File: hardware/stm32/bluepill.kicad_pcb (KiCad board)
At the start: 2 copper layers, 99.1 x 99.1 mm, 71 parts, among them J1 LCD, J10 Screw_Terminal_01x02, J11 Screw_Terminal_01x02, J12 Screw_Terminal_01x02, J13 Screw_Terminal_01x02, J14 RTC, J15 Screw_Terminal_01x02, J16 Conn_01x02_Male, J17 ESP-01, J18 USART1, J19 Buttons, J2 SD Card, J3 Radio, J4 Inside, J5 Outside, J6 Screw_Terminal_01x02, J7 Conn_01x02, J8 Screw_Terminal_01x02, J9 Screw_Terminal_01x02, Q1 Q_NMOS_GSD, Q2 Q_NMOS_GSD, Q3 Q_NMOS_GSD, Q4 Q_NMOS_GSD, Q5 Q_NMOS_GSD, Q6 Q_NMOS_GSD, U1 PC817, U10 PC817, U11 PC817, U12 LM1117-3.3, U2 24LC512, U3 bluepill, U4 PC817, U5 PC817, U6 PC817, U7 PC817, U8 PC817, U9 PC817

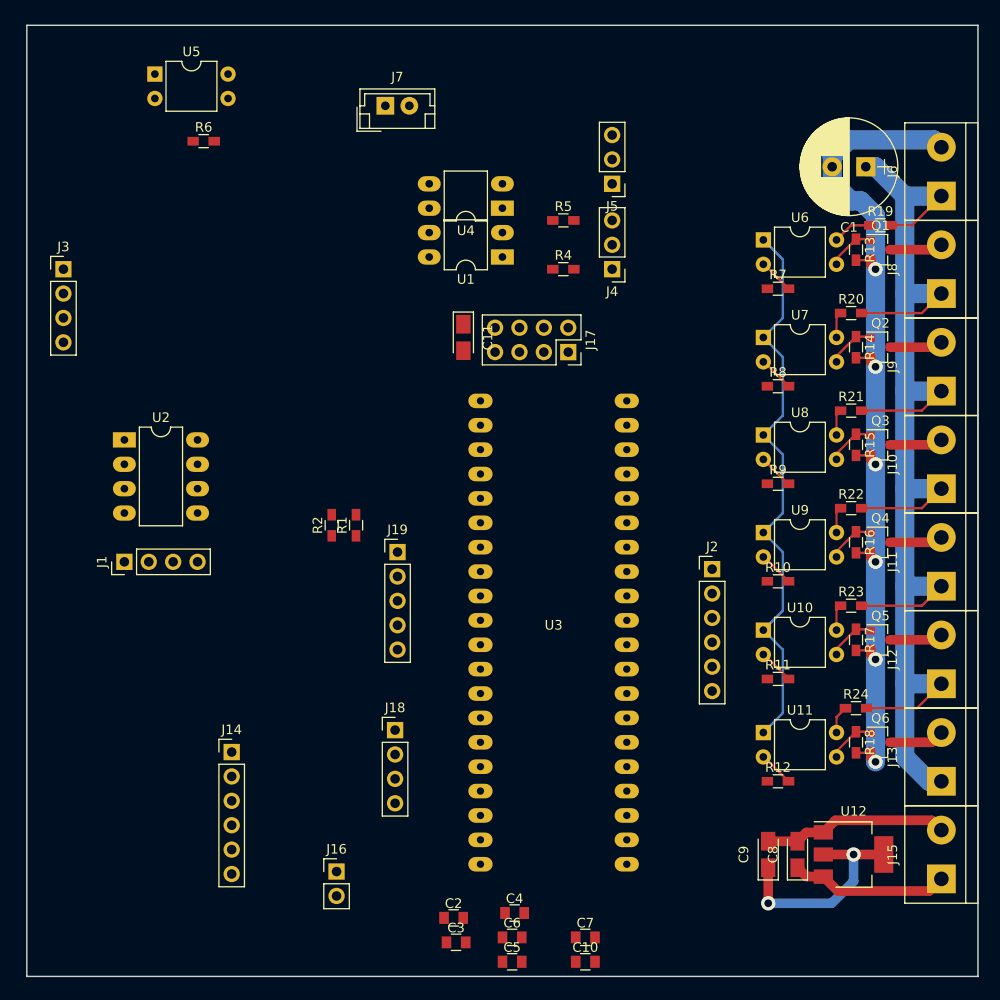
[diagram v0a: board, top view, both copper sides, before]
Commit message: bluepill PCB progress
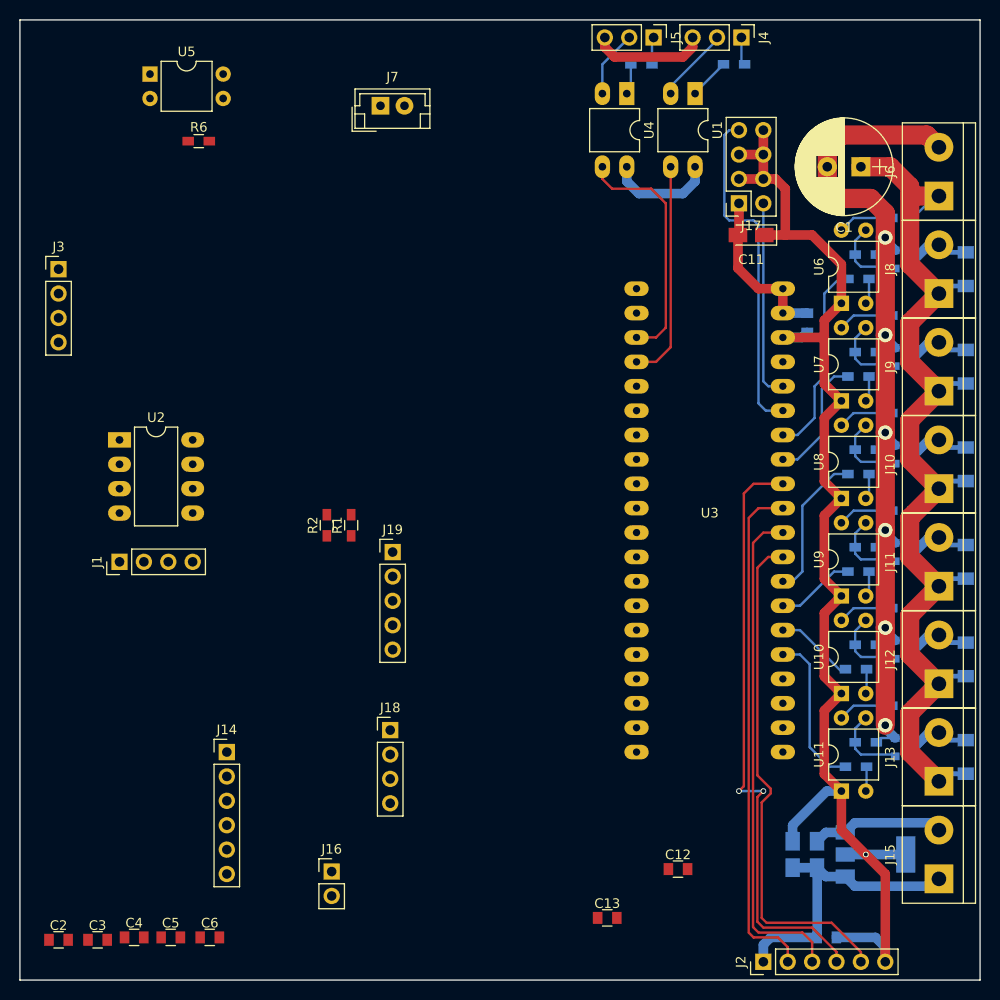
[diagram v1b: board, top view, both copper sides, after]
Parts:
- added C12: 100n, Capacitors_SMD:C_0805, F.Cu at (113.5, 123.4)
- added C13: 100n, Capacitors_SMD:C_0805, F.Cu at (106.2, 128.5)
- added D1: 1N4148, Diodes_SMD:D_MiniMELF, B.Cu at (143.5, 61.0)
- added D2: 1N4148, Diodes_SMD:D_MiniMELF, B.Cu at (143.5, 71.1)
- added D3: 1N4148, Diodes_SMD:D_MiniMELF, B.Cu at (143.5, 81.3)
- added D4: 1N4148, Diodes_SMD:D_MiniMELF, B.Cu at (143.5, 91.4)
- added D5: 1N4148, Diodes_SMD:D_MiniMELF, B.Cu at (143.5, 101.6)
- added D6: 1N4148, Diodes_SMD:D_MiniMELF, B.Cu at (143.5, 111.8)
- C10, C7, C8, C9, R10, R11, R12, R13, R14, R15, R16, R17, R18, R19, R20, R21, R22, R23, R24, R4, R5, R7, R8, R9, U12: moved to B.Cu
- J15: value Screw_Terminal_01x02 -> +5V
- Q1, Q2, Q3, Q4, Q5, Q6: value Q_NMOS_GSD -> IRLML2502; moved to B.Cu
- moved C7 68.1 mm to (127.0, 66.5), turned to 90 degrees
- moved J2 41.2 mm to (122.4, 133.1), turned to 90 degrees
- moved C2 41.2 mm to (49.0, 130.8)
- moved C4 39.7 mm to (56.9, 130.6)
- moved C3 37.3 mm to (53.1, 130.8)
- moved C5 35.7 mm to (60.7, 130.6)
- moved C11 31.8 mm to (121.2, 57.4), turned to 180 degrees
- moved C6 31.5 mm to (64.8, 130.6)
- moved R4 27.8 mm to (119.4, 39.6)
- moved J4 27.6 mm to (120.1, 36.8), turned to 270 degrees
- moved U1 26.3 mm to (115.3, 42.7), turned to 270 degrees
- moved C10 25.3 mm to (129.0, 130.6), turned to 180 degrees
- moved J17 23.6 mm to (119.9, 54.1), turned to 180 degrees
- moved U3 20.0 mm to (116.8, 85.9)
- moved R5 18.2 mm to (109.7, 39.6)
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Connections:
- J15 pad 1: +5V -> GND
- J15 pad 2: GND -> +5V
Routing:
- net +3V3: track 82.4 -> 148.7 mm, vias 2 -> 1
- net /MCU/MOSI: track 0.00 -> 62.7 mm, vias 0 -> 2
- net /MCU/MISO: track 0.00 -> 53.4 mm
- net /MCU/CS: track 0.00 -> 53.4 mm
- net /MCU/SCK: track 0.00 -> 52.4 mm
- net GND: track 19.4 -> 60.8 mm
- net /MCU/ESP_RX: track 0.00 -> 35.5 mm
- net /MCU/LOOP_O: track 0.00 -> 25.3 mm
- net /MCU/LOOP_I: track 0.00 -> 23.0 mm
- net Net-(R7-Pad1): track 0.00 -> 21.5 mm
- net /MCU/ESP_TX: track 0.00 -> 20.8 mm
- net +12V: track 143.4 -> 126.5 mm
- net Net-(R12-Pad1): track 0.00 -> 16.4 mm
- net Net-(R9-Pad1): track 0.00 -> 15.4 mm
- net Net-(R8-Pad1): track 0.00 -> 13.2 mm
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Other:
- board size 99.1 x 99.1 mm -> 100 x 100 mm
- net class 12V added: clearance 0.2, trace_width 2, via_dia 2, via_drill 0.8
- net class 3.3V: trace_width 0.5 -> 1
- net class 5V: trace_width 0.5 -> 1
- net class Default: trace_width 0.25 -> 0.254
- net class GND: trace_width 0.5 -> 1
- net class Strong added: clearance 0.2, trace_width 1, via_dia 0.6, via_drill 0.4
